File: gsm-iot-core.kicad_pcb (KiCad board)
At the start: 2 copper layers, 25.4 x 68.6 mm, 93 parts, among them J1 MICRO_SD_HINGE - Micro SD soc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, P1 CONN_01X17, P2 CONN_01X17, P3 Chip anten, Q1 2SC1815, Q2 2SC1815, SW1 SW_PUSH, SW2 SW_PUSH, U1 MP2365DN, U2 LP2985-50DBVR, U3 STM32F405RGTx, U4 MMA7660, U5 SIM800C, U6 SIM HOLD - PPSS-6P, X1 CRYSTAL-24M, Y1 32.768MHz

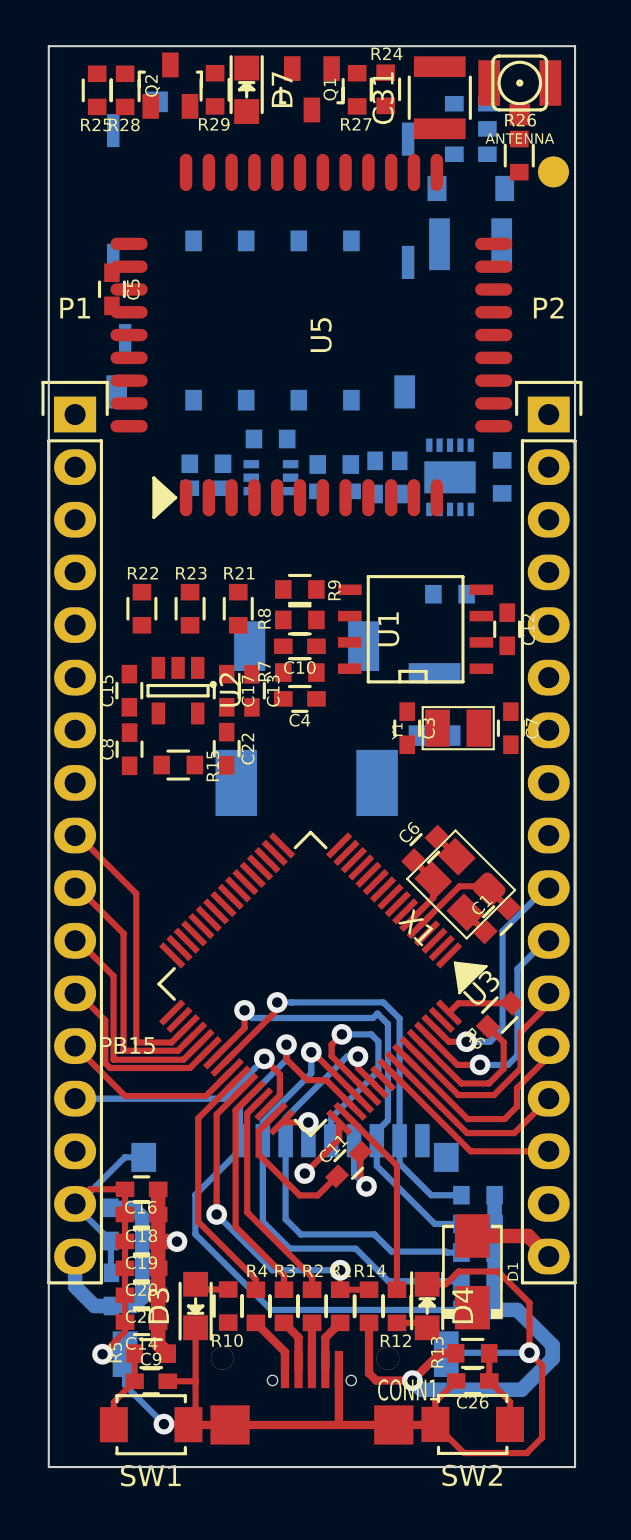
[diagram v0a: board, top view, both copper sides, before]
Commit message: completed connect tracks
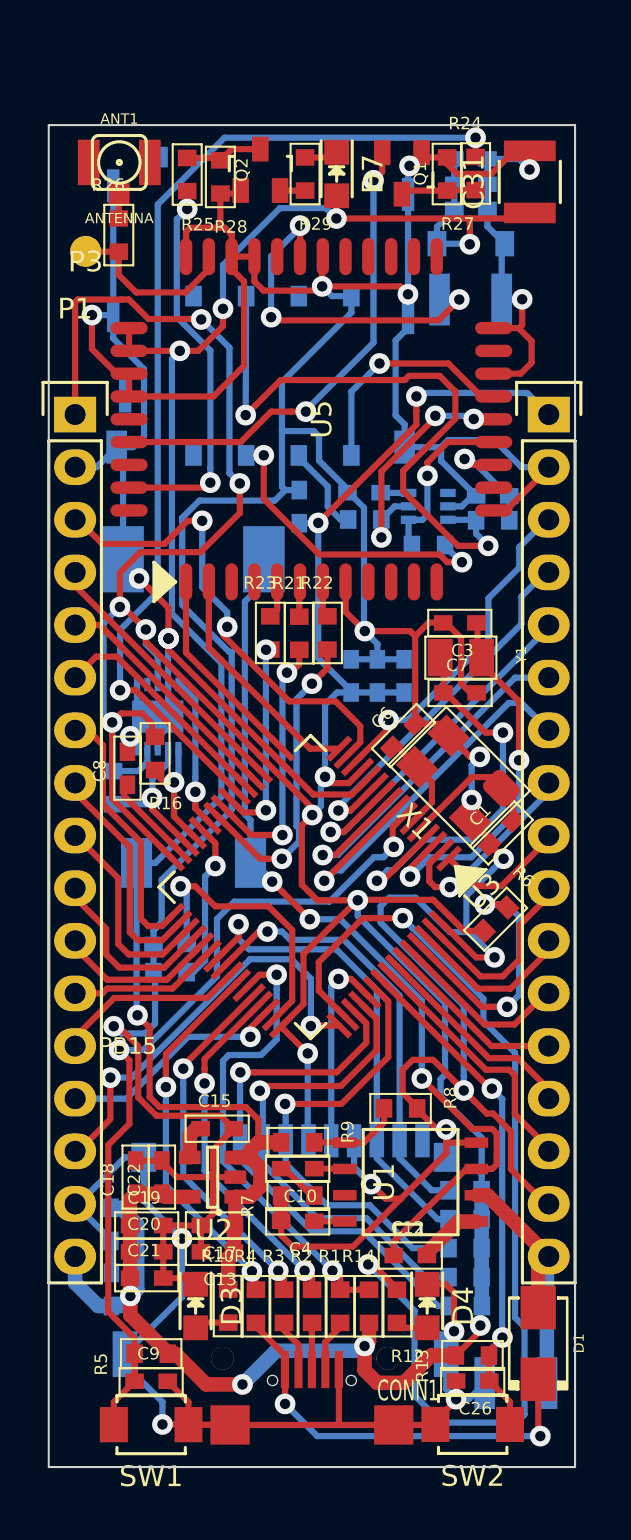
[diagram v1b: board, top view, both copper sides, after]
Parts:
- removed C5: 100nF, lib:C_0603
- C11, C14, C16, R15: moved to B.Cu
- R16: moved to F.Cu
- X1: footprint lib:Crystal_SMD_3225_4Pads -> lib:Crystal_SMD_5032_4Pads
- moved C2 33.0 mm to (171.1, 125.5), turned to 180 degrees
- moved C14 32.8 mm to (163.2, 91.4), turned to 90 degrees
- moved C12 30.6 mm to (166.0, 119.3), turned to 0 degrees
- moved C16 27.3 mm to (164.5, 91.4), turned to 90 degrees
- moved C13 27.1 mm to (156.7, 119.2), turned to 180 degrees
- moved R9 26.7 mm to (160.6, 113.9)
- moved U1 26.7 mm to (166.1, 115.8)
- moved C17 25.8 mm to (156.7, 117.9), turned to 180 degrees
- moved R7 25.2 mm to (160.6, 116.4)
- moved C4 25.2 mm to (160.6, 117.7)
- moved C10 25.2 mm to (160.6, 115.1)
- moved R8 24.1 mm to (165.6, 112.2), turned to 0 degrees
- moved U2 23.5 mm to (156.5, 115.5), turned to 180 degrees
- moved P3 22.9 mm to (150.4, 70.9)
- moved C15 21.6 mm to (156.7, 113.2), turned to 0 degrees
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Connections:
- D5 pad 1: Net-(D5-Pad1) -> (no net)
- J1 pad 9: Net-(J1-Pad9) -> (no net)
- U1 pad 7: Net-(U1-Pad7) -> (no net)
- U4 pad 2: Net-(U4-Pad2) -> (no net)
- U5 pad 10: Net-(U5-Pad10) -> (no net)
- U5 pad 11: Net-(U5-Pad11) -> (no net)
- U5 pad 12: Net-(U5-Pad12) -> (no net)
- U5 pad 14: Net-(U5-Pad14) -> (no net)
- U5 pad 20: Net-(U5-Pad20) -> (no net)
- U5 pad 22: Net-(U5-Pad22) -> (no net)
- U5 pad 23: Net-(U5-Pad23) -> (no net)
- U5 pad 24: Net-(U5-Pad24) -> (no net)
- U5 pad 25: Net-(U5-Pad25) -> (no net)
- U5 pad 26: Net-(U5-Pad26) -> (no net)
- U5 pad 29: Net-(U5-Pad29) -> (no net)
- U5 pad 3: Net-(U5-Pad3) -> (no net)
- U5 pad 38: Net-(U5-Pad38) -> (no net)
- U5 pad 4: Net-(U5-Pad4) -> (no net)
- U5 pad 40: Net-(U5-Pad40) -> (no net)
- U5 pad 42: Net-(U5-Pad42) -> (no net)
- U5 pad 9: Net-(U5-Pad9) -> (no net)
- U6 pad 6: Net-(U6-Pad6) -> (no net)
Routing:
- net GND: track 78.7 -> 376.7 mm, vias 4 -> 23
- net +3V3: track 51.5 -> 196.8 mm, vias 3 -> 15
- net VDD: track 0.00 -> 90.6 mm, vias 0 -> 5
- net PA7_PWRKEY: track 0.00 -> 49.5 mm, vias 0 -> 2
- net Net-(C12-Pad1): track 0.00 -> 43.3 mm, vias 0 -> 3
- net PA15_LED: track 9.44 -> 49.8 mm, vias 0 -> 2
- net /RST: track 3.84 -> 40.4 mm, vias 0 -> 2
- net Net-(D5-Pad3): track 0.00 -> 30.9 mm, vias 0 -> 2
- net PA1: track 0.00 -> 23.3 mm, vias 0 -> 2
- net SIM800C_PWRKEY: track 0.00 -> 23.2 mm, vias 0 -> 2
- net PB3_BUTTON: track 3.84 -> 24.5 mm, vias 0 -> 2
- net PC0: track 0.00 -> 20.0 mm, vias 0 -> 1
- net Net-(C7-Pad1): track 0.00 -> 19.9 mm, vias 0 -> 2
- net SIM800C_NETLIGHT: track 0.00 -> 19.0 mm, vias 0 -> 2
- net PC1: track 0.00 -> 18.8 mm, vias 0 -> 1
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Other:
- board size 25.4 x 68.6 mm -> 25.4 x 64.8 mm
- net class Default: clearance 0.1 -> 0.254
- rule trace_clearance: 0.1 -> 0.254
